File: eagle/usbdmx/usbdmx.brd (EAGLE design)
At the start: 63.2 x 50.2 mm, 33 parts, among them IC1 MAX3468CSA, IC2 MAX3468CSA, Q1 16MHz

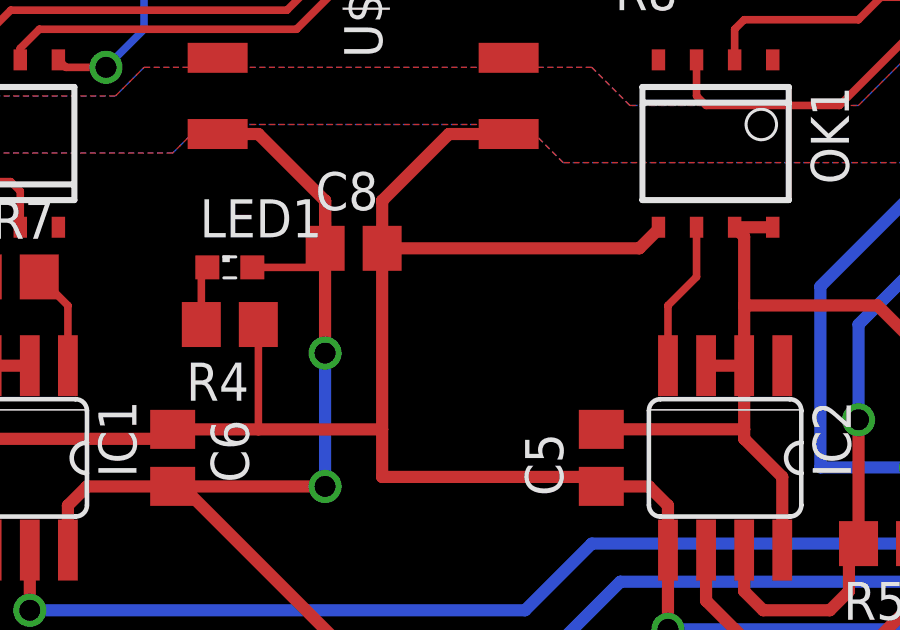
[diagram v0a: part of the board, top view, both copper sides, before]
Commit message: fix minor errors
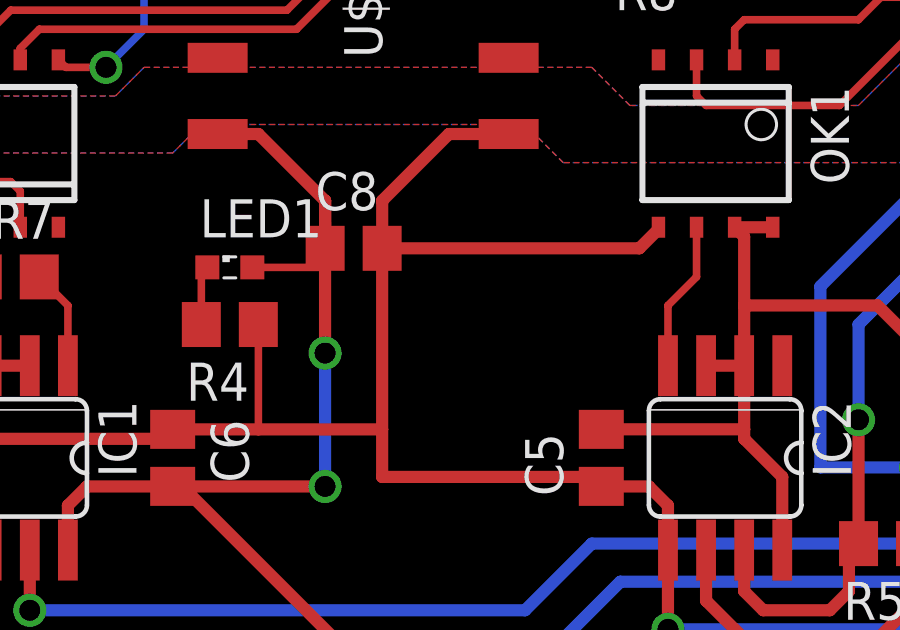
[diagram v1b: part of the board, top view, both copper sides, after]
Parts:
- C4, C5, C6, C7: value (none) -> 100n
- C8: value (none) -> 4,7µ
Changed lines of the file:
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@@
 <element name="U$1" library="adafruit" package="TQFP44" value="ATMEGA32U4-AU" x="33.9725" y="39.37"/>
 <element name="X1" library="con-usb-3" package="USB-B-SMT" value="" x="8.5725" y="40.64"/>
-<element name="C4" library="rcl" package="C0805" value="" x="20.0025" y="38.735"/>
-<element name="C5" library="rcl" package="C0805" value="" x="30.48" y="8.255" rot="R90"/>
-<element name="C6" library="rcl" package="C0805" value="" x="16.1925" y="8.255" rot="R270"/>
+<element name="C4" library="rcl" package="C0805" value="100n" x="20.0025" y="38.735"/>
+<element name="C5" library="rcl" package="C0805" value="100n" x="30.48" y="8.255" rot="R90"/>
+<element name="C6" library="rcl" package="C0805" value="100n" x="16.1925" y="8.255" rot="R270"/>
 <element name="JP1" library="pinhead" package="2X03SMD" value="ICSP" x="9.2075" y="29.21" rot="R270"/>
-<element name="C7" library="rcl" package="C0805" value="" x="27.6225" y="45.4025" rot="R180"/>
+<element name="C7" library="rcl" package="C0805" value="100n" x="27.6225" y="45.4025" rot="R180"/>
 <element name="DMXOUT" library="con-neutrik_ag" package="NC3FAH2" value="NC3FAH2" x="49.8475" y="37.465" rot="R270">
 <attribute name="OC_NEWARK" value="27B4208" x="49.8475" y="37.465" size="1.778" layer="27" rot="R270" display="off"/>
@@
 </element>
 <element name="U$2" library="murata-dcdc" package="SMT" value="NTE0505SNTE0505MEC" x="22.5425" y="22.86"/>
-<element name="C8" library="rcl" package="C0805" value="" x="22.225" y="15.24"/>
+<element name="C8" library="rcl" package="C0805" value="4,7µ" x="22.225" y="15.24"/>
 <element name="R5" library="rcl" package="R0805" value="120" x="40.005" y="5.3975" rot="R180"/>
 <element name="OK1" library="optocoupler" package="SO-8" value="6N137SO-8" x="34.29" y="18.7325" rot="R270"/>
@@
 <contactref element="DMXOUT" pad="1"/>
 <contactref element="DMXOUT" pad="G"/>
-<contactref element="U$2" pad="8"/>
-<contactref element="C8" pad="2"/>
 <contactref element="C5" pad="1"/>
-<wire x1="27.3925" y1="19.05" x2="25.4" y2="19.05" width="0.4064" layer="1"/>
-<wire x1="25.4" y1="19.05" x2="23.1775" y2="16.8275" width="0.4064" layer="1"/>
-<wire x1="23.1775" y1="16.8275" x2="23.1775" y2="16.83" width="0.4064" layer="1"/>
-<wire x1="23.1775" y1="16.83" x2="23.175" y2="15.24" width="0.4064" layer="1"/>
 <contactref element="OK1" pad="5"/>
 <contactref element="OK2" pad="3"/>
-<wire x1="23.175" y1="15.24" x2="31.75" y2="15.24" width="0.4064" layer="1"/>
 <wire x1="31.75" y1="15.24" x2="32.385" y2="15.875" width="0.4064" layer="1"/>
 <wire x1="32.385" y1="15.875" x2="32.385" y2="15.9425" width="0.4064" layer="1"/>
 <wire x1="30.48" y1="7.305" x2="30.165" y2="7.62" width="0.4064" layer="1"/>
 <wire x1="30.165" y1="7.62" x2="23.175" y2="7.62" width="0.4064" layer="1"/>
-<wire x1="23.175" y1="9.205" x2="23.175" y2="15.24" width="0.4064" layer="1"/>
 <wire x1="51.435" y1="41.275" x2="51.7625" y2="41.275" width="0.4064" layer="16"/>
 <wire x1="51.7625" y1="41.275" x2="56.2025" y2="45.715" width="0.4064" layer="16"/>
@@
 <contactref element="IC1" pad="2"/>
 <wire x1="10.16" y1="11.3284" x2="11.43" y2="11.3284" width="0.4064" layer="1"/>
-<contactref element="R4" pad="1"/>
-<wire x1="19.0475" y1="12.7" x2="19.05" y2="12.7" width="0.254" layer="1"/>
 <wire x1="19.05" y1="12.7" x2="19.05" y2="9.205" width="0.254" layer="1"/>
 <polygon width="0.4064" layer="1" isolate="0.6096" orphans="yes">
@@
 <vertex x="0.9525" y="0.9525"/>
 </polygon>
+<contactref element="R4" pad="1"/>
+<contactref element="C8" pad="2"/>
+<contactref element="U$2" pad="8"/>
+<wire x1="27.3925" y1="19.05" x2="25.4" y2="19.05" width="0.4064" layer="1"/>
+<wire x1="25.4" y1="19.05" x2="23.1775" y2="16.8275" width="0.4064" layer="1"/>
+<wire x1="23.1775" y1="16.8275" x2="23.1775" y2="15.2425" width="0.4064" layer="1"/>
+<wire x1="23.1775" y1="15.2425" x2="23.175" y2="15.24" width="0.4064" layer="1"/>
+<wire x1="23.175" y1="15.24" x2="23.175" y2="9.205" width="0.4064" layer="1"/>
+<wire x1="31.75" y1="15.24" x2="23.175" y2="15.24" width="0.4064" layer="1"/>
 </signal>
 <signal name="N$20">
